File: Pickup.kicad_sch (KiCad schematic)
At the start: 36 parts, among them U401 PCM1808, U402 PCM1808, U403 PCM1808

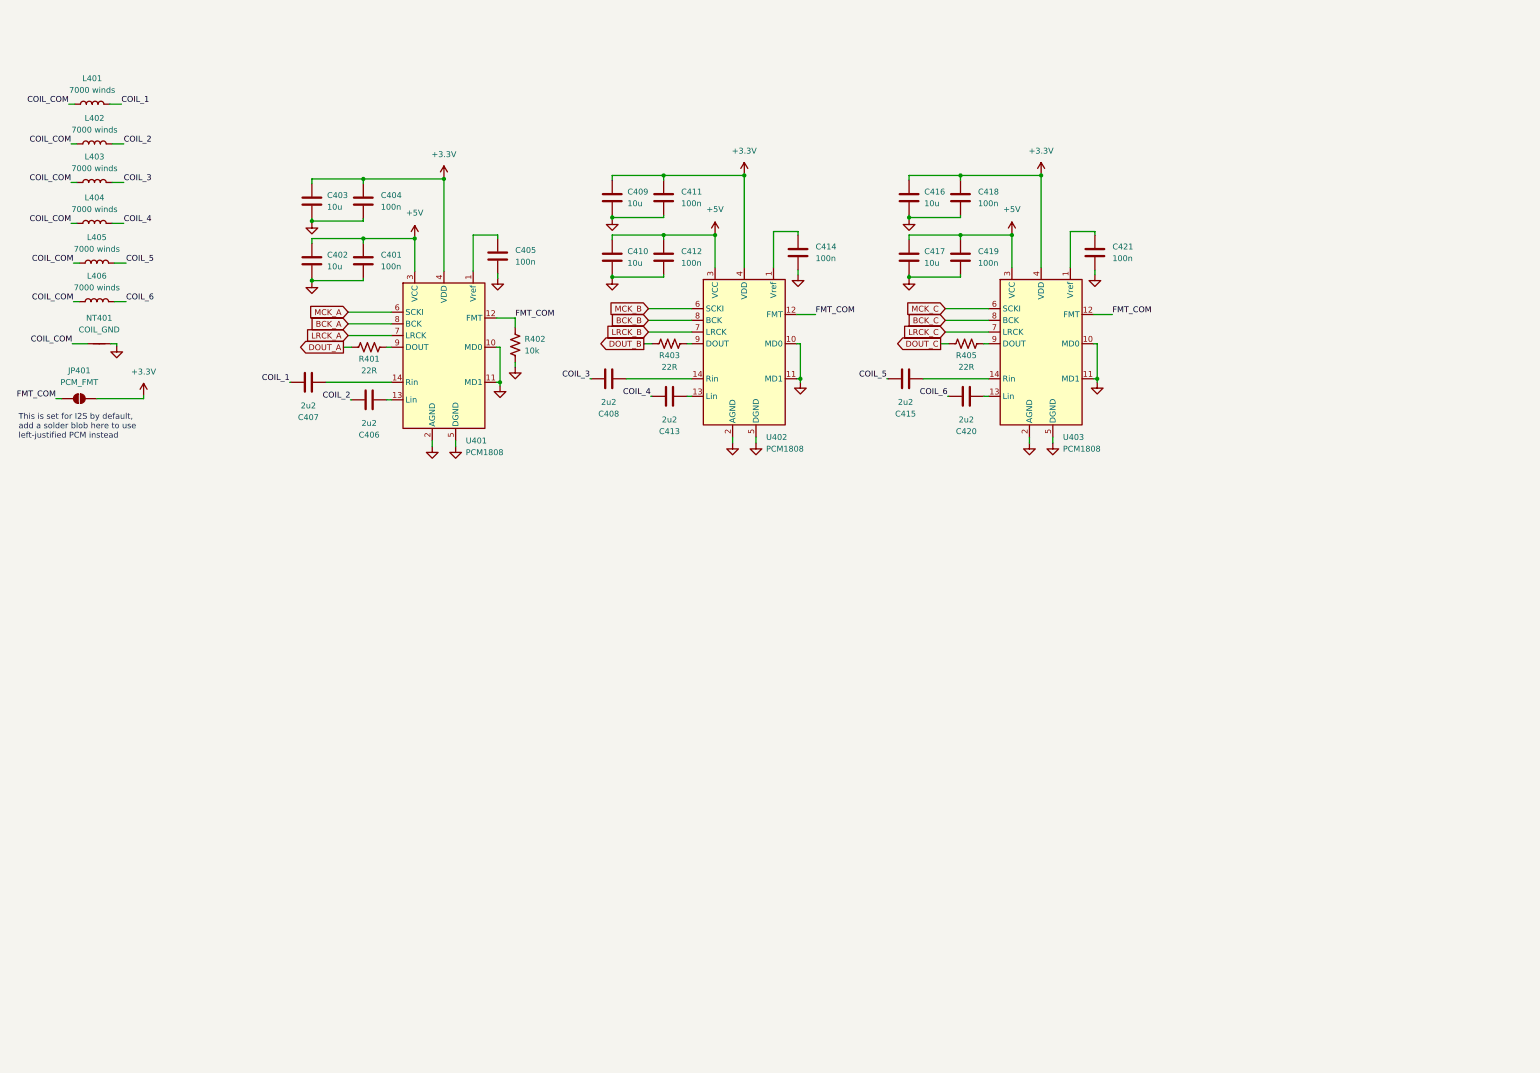
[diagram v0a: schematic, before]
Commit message: op amp input stage
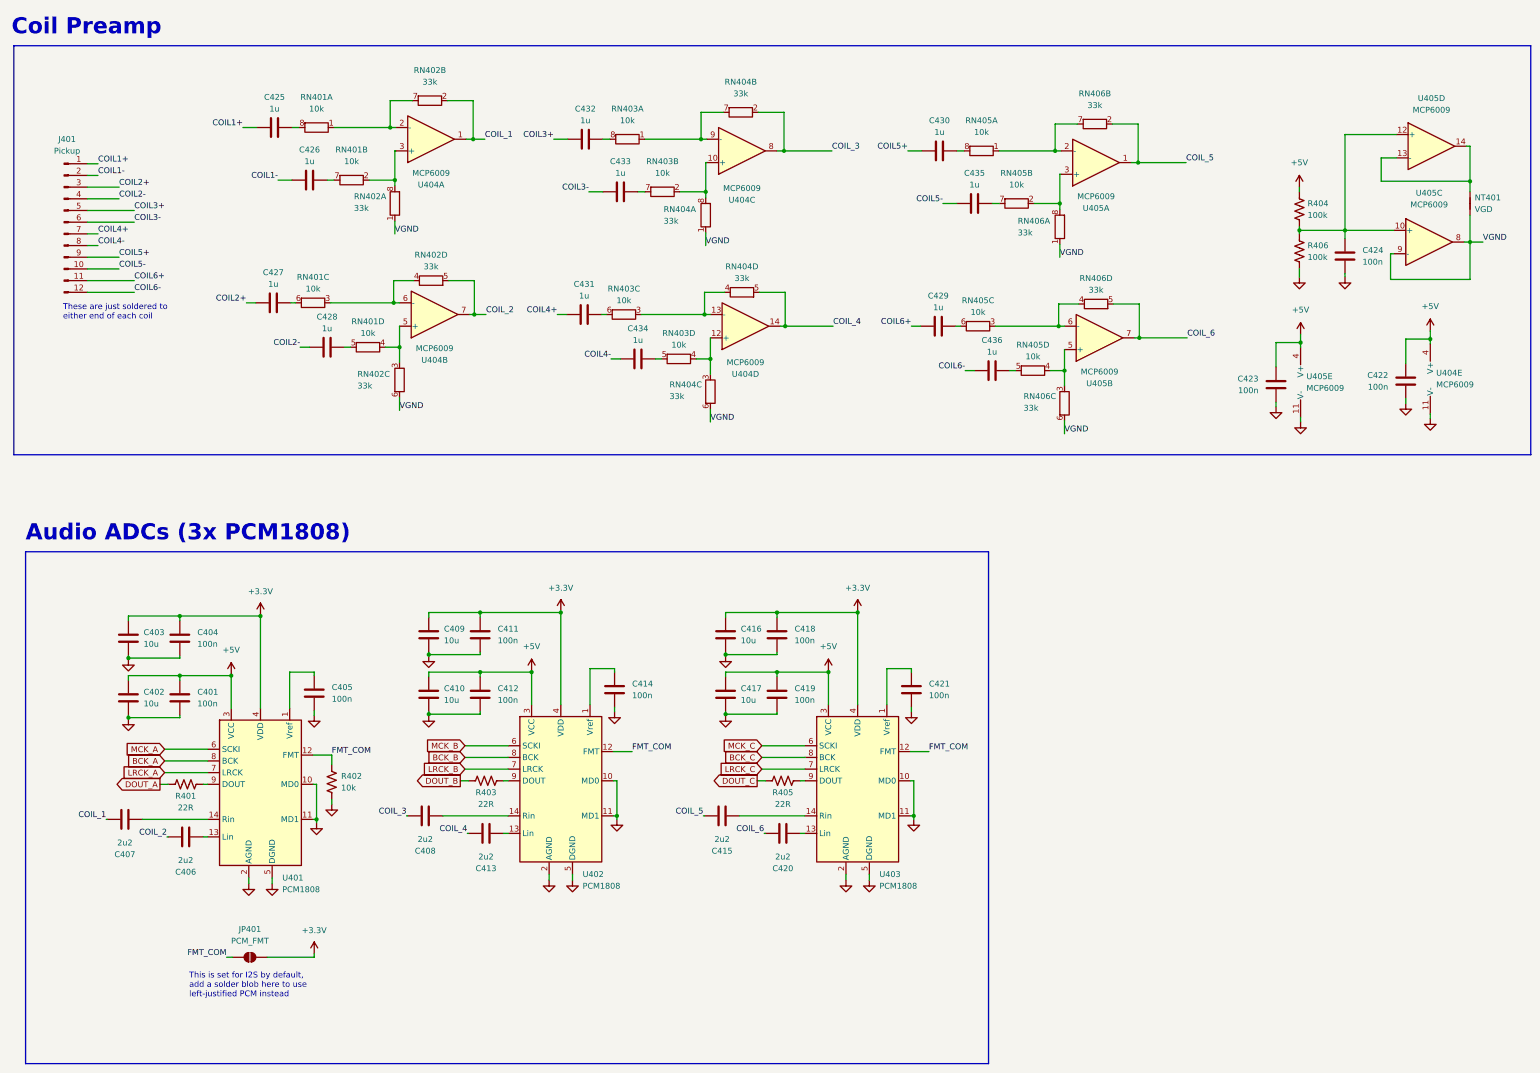
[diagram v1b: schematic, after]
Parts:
- removed L401, L402, L403, L404, L405, L406: 7000 winds, Inductor_THT:L_Radial_L8.0mm_W8.0mm_P5.00mm_Neosid_SD8, symbol Device:L
- added C422, C423, C424: 100n, Capacitor_SMD:C_0805_2012Metric, symbol Device:C
- added C425, C426, C427, C428, C429, C430, C431, C432, C433, C434, C435, C436: 1u, Capacitor_SMD:C_0805_2012Metric, symbol Device:C
- added J401: Pickup, Connector_JST:JST_PH_B12B-PH-K_1x12_P2.00mm_Vertical, symbol Connector:Conn_01x12_Pin
- added R404, R406: 100k, Resistor_SMD:R_0805_2012Metric, symbol Device:R_US
- added RN401, RN403, RN405: 10k, Resistor_SMD:R_Array_Concave_4x0603, symbol Device:R_Pack04_Split
- added RN402, RN404, RN406: 33k, Resistor_SMD:R_Array_Concave_4x0603, symbol Device:R_Pack04_Split
- added U404, U405: MCP6009, Package_SO:TSSOP-14_4.4x5mm_P0.65mm, symbol Amplifier_Operational:MCP604
- NT401: value COIL_GND -> VGD
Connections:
- net +5V: now also C422.1, C423.1, R404.1, U404.4 (V+), U405.4 (V+)
- net COIL_1: now also RN402.2 (R2.1), U404.1
- net COIL_2: now also RN402.5 (R4.2), U404.7
- net COIL_3: now also RN404.2 (R2.1), U404.8
- net COIL_4: now also RN404.5 (R4.2), U404.14
- net COIL_5: now also RN406.2 (R2.1), U405.1
- net COIL_6: now also RN406.5 (R4.2), U405.7
- net GND: now also C422.2, C423.2, C424.2, R406.2, U404.11 (V-), U405.11 (V-); no longer NT401.2
- net COIL_COM renamed VGND
- net VGND: now also RN402.1 (R1.1), RN402.6 (R3.2), RN404.1 (R1.1), RN404.6 (R3.2), RN406.1 (R1.1), RN406.6 (R3.2), U405.8, U405.9 (-)
- new net: C424.1, R404.2, R406.1, U405.10 (+), U405.12 (+)
- new net: RN401.1 (R1.1), RN402.7 (R2.2), U404.2 (-)
- new net: C431.2, RN403.6 (R3.2)
- new net: RN401.4 (R4.1), RN402.3 (R3.1), U404.5 (+)
- new net: RN401.3 (R3.1), RN402.4 (R4.1), U404.6 (-)
- new net: RN403.2 (R2.1), RN404.8 (R1.2), U404.10 (+)
- new net: C433.2, RN403.7 (R2.2)
- new net: C427.2, RN401.6 (R3.2)
- new net: C428.2, RN401.5 (R4.2)
- new net: RN405.1 (R1.1), RN406.7 (R2.2), U405.2 (-)
- new net: NT401.2, U405.13 (-), U405.14
- new net: C426.2, RN401.7 (R2.2)
- new net: RN401.2 (R2.1), RN402.8 (R1.2), U404.3 (+)
- new net: C429.2, RN405.6 (R3.2)
- new net: RN405.3 (R3.1), RN406.4 (R4.1), U405.6 (-)
- new net: C435.2, RN405.7 (R2.2)
- new net: RN403.3 (R3.1), RN404.4 (R4.1), U404.13 (-)
- new net: RN403.4 (R4.1), RN404.3 (R3.1), U404.12 (+)
- new net: C434.2, RN403.5 (R4.2)
- new net: RN405.2 (R2.1), RN406.8 (R1.2), U405.3 (+)
- new net: C432.2, RN403.8 (R1.2)
- new net: RN403.1 (R1.1), RN404.7 (R2.2), U404.9 (-)
- new net: RN405.4 (R4.1), RN406.3 (R3.1), U405.5 (+)
- new net: C436.2, RN405.5 (R4.2)
- new net: C425.2, RN401.8 (R1.2)
- new net: C430.2, RN405.8 (R1.2)
- new net COIL1+: C425.1, J401.1 (Pin_1)
- new net COIL1-: C426.1, J401.2 (Pin_2)
- new net COIL2+: C427.1, J401.3 (Pin_3)
- new net COIL2-: C428.1, J401.4 (Pin_4)
- new net COIL3+: C432.1, J401.5 (Pin_5)
- new net COIL3-: C433.1, J401.6 (Pin_6)
- new net COIL4+: C431.1, J401.7 (Pin_7)
- new net COIL4-: C434.1, J401.8 (Pin_8)
- new net COIL5+: C430.1, J401.9 (Pin_9)
- new net COIL5-: C435.1, J401.10 (Pin_10)
- new net COIL6+: C429.1, J401.11 (Pin_11)
- new net COIL6-: C436.1, J401.12 (Pin_12)
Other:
- note added: "Audio ADCs (3x PCM1808)"
- note added: "Coil Preamp"
- note added: "These are just soldered to either end of each coil"
- moved on the sheet: C401, C402, C403, C404, C405, C406, C407, C408, C409, C410, C411, C412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
